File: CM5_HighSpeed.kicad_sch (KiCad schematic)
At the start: 5 parts, among them J10 690-019-298-412, U20 RT9742SNGV

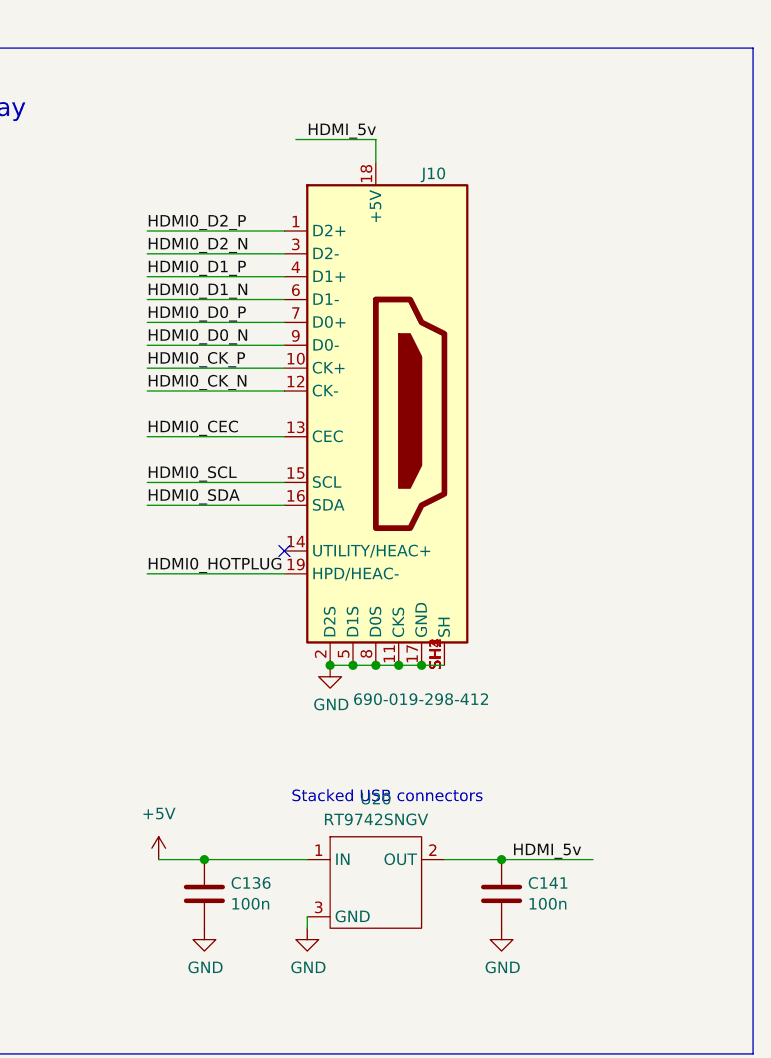
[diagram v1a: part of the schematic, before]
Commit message: end route
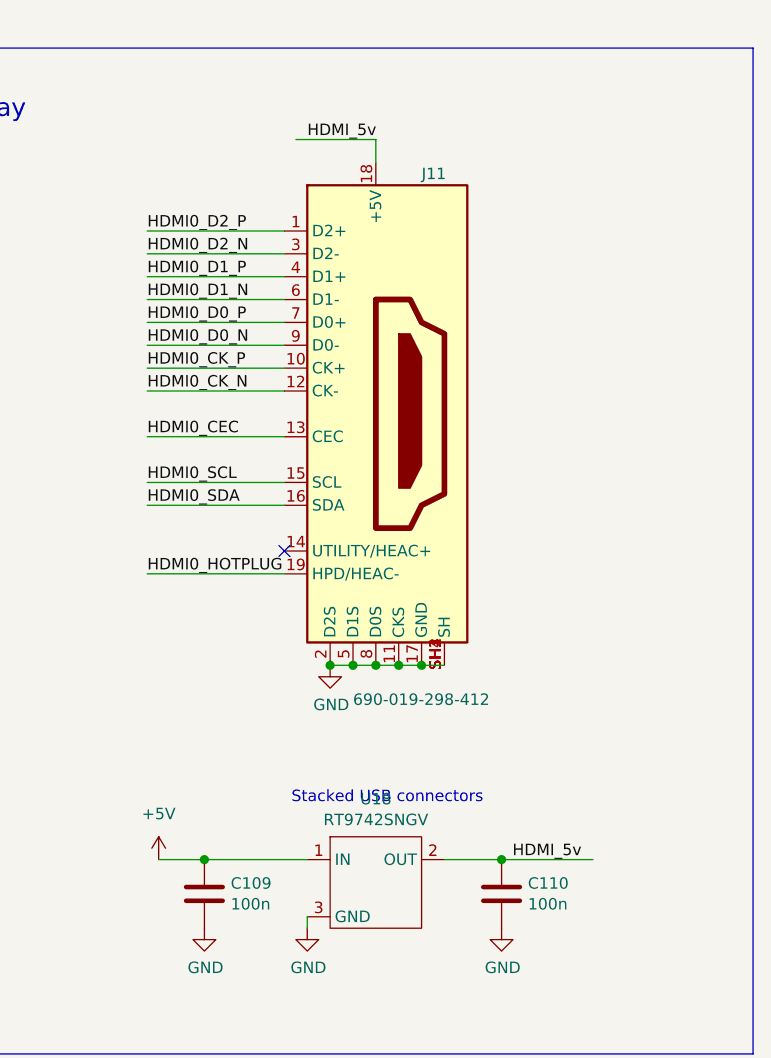
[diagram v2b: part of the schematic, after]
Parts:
- renumbered C136 to C109, C141 to C110, J10 to J11, U20 to U18
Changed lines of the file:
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@@
 		(on_board yes)
 		(dnp no)
-		(property "Reference" "J10"
+		(property "Reference" "J11"
 			(at 224.79 58.42 0)
 			(effects
@@
 			(project "CM5IO"
 				(path "/dd07ab80-a59c-44f4-ac7d-849e21e1384e/5e5501ac-41c8-4cac-b3fc-c2c46c035d54"
-					(reference "J10")
+					(reference "J11")
 					(unit 1)
 				)
@@
 		(on_board yes)
 		(dnp no)
-		(property "Reference" "C141"
+		(property "Reference" "C110"
 			(at 236.601 137.2616 0)
 			(effects
@@
 			(project "CM5IO"
 				(path "/dd07ab80-a59c-44f4-ac7d-849e21e1384e/5e5501ac-41c8-4cac-b3fc-c2c46c035d54"
-					(reference "C141")
+					(reference "C110")
 					(unit 1)
 				)
@@
 		(on_board yes)
 		(dnp no)
-		(property "Reference" "C136"
+		(property "Reference" "C109"
 			(at 203.581 137.2616 0)
 			(effects
@@
 			(project "CM5IO"
 				(path "/dd07ab80-a59c-44f4-ac7d-849e21e1384e/5e5501ac-41c8-4cac-b3fc-c2c46c035d54"
-					(reference "C136")
+					(reference "C109")
 					(unit 1)
 				)
@@
 		(on_board yes)
 		(dnp no)
-		(property "Reference" "U20"
+		(property "Reference" "U18"
 			(at 219.71 127.889 0)
 			(effects
@@
 			(project "CM5IO"
 				(path "/dd07ab80-a59c-44f4-ac7d-849e21e1384e/5e5501ac-41c8-4cac-b3fc-c2c46c035d54"
-					(reference "U20")
-					(unit 1)
-				)
+					(reference "U18")
+					(unit 1)
+				)
